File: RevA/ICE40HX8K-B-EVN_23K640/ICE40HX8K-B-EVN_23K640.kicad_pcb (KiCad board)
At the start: 2 copper layers, 50.8 x 17.4 mm, 19 parts, among them J1 2x20_Socket, U0 23K640, U1 23K640, U2 23K640, U3 23K640, U4 23K640, U5 23K640, U6 23K640, U7 23K640

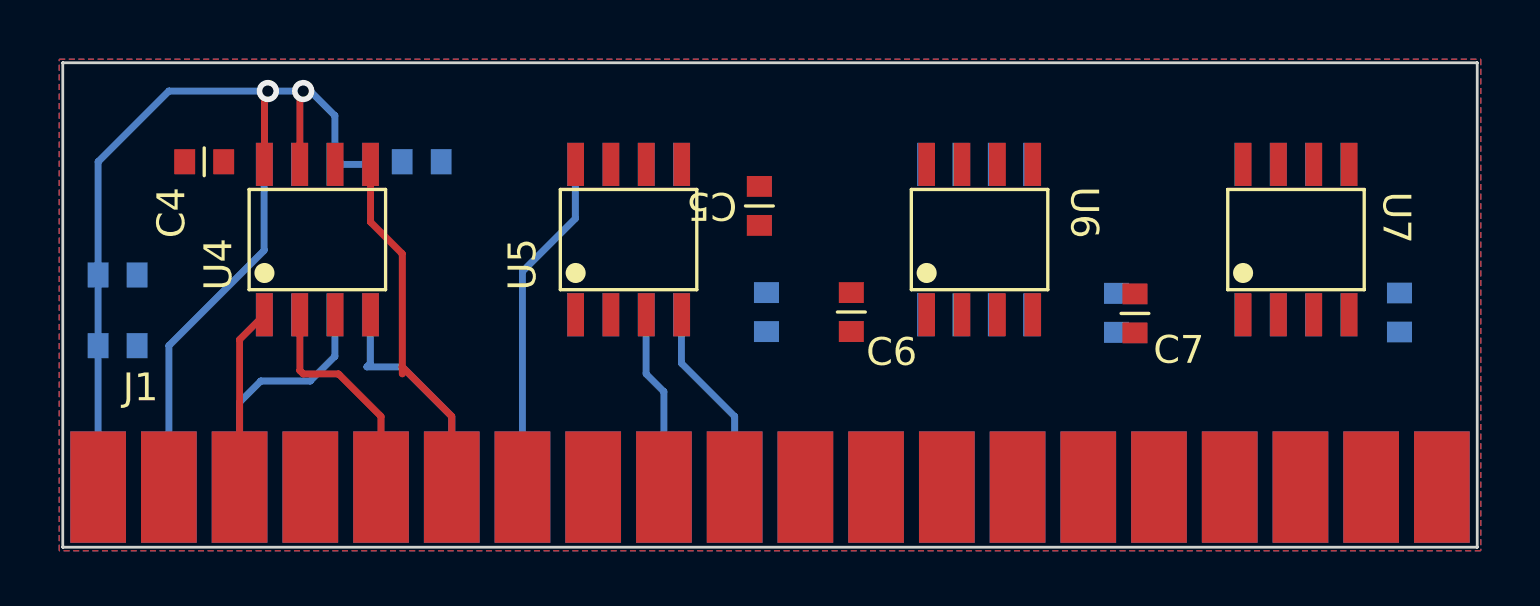
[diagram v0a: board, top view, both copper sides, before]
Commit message: routed
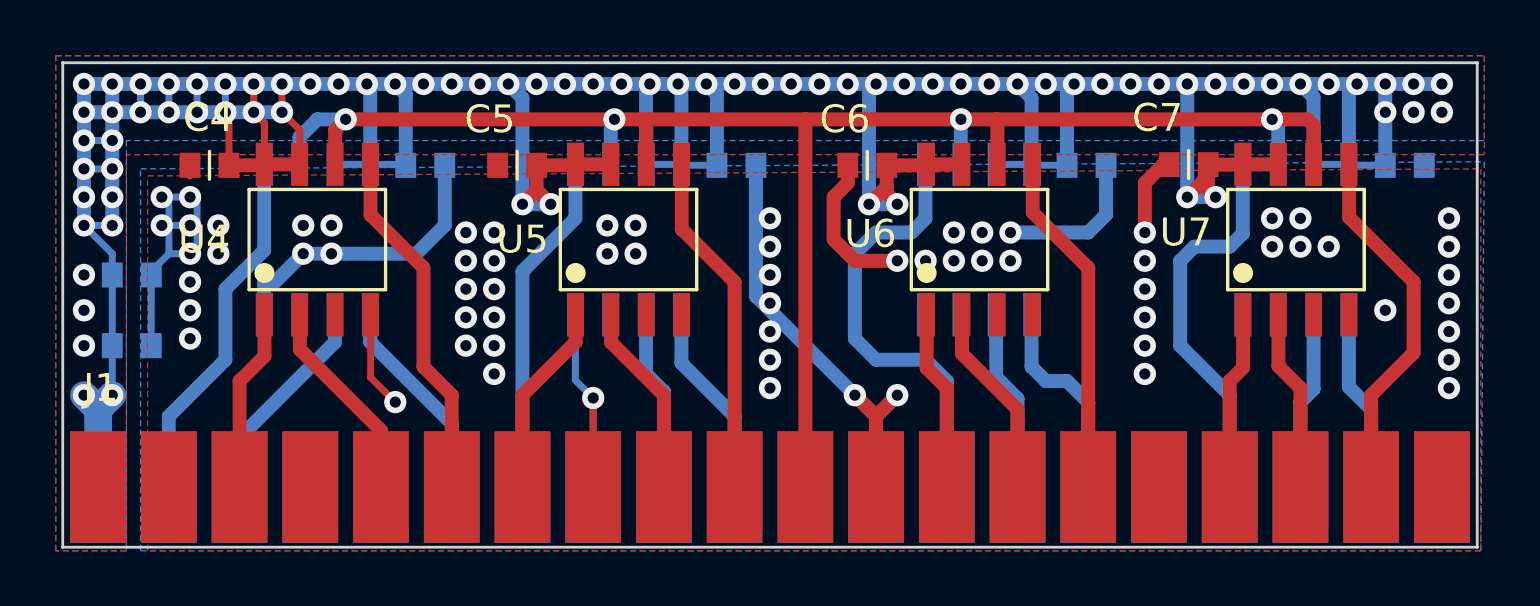
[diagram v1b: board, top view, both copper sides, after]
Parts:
- moved C5 9.65 mm to (80.4, 112.9), turned to 0 degrees
- moved C7 6.17 mm to (104.5, 112.9), turned to 0 degrees
- moved C3 6.05 mm to (113.7, 112.9), turned to 180 degrees
- moved C2 6.01 mm to (102.2, 112.9), turned to 180 degrees
- moved C1 5.98 mm to (89.7, 112.9), turned to 180 degrees
- moved C6 5.97 mm to (93.0, 112.9), turned to 0 degrees
- moved C8 0.51 mm to (67.9, 116.8)
- moved C9 0.51 mm to (67.9, 119.4)
- moved C4 0.23 mm to (69.3, 112.9)
- moved C0 0.18 mm to (78.5, 112.9)
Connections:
- J1 pad 25: /SI_6 -> /nCS_6
- J1 pad 26: /nCS_2 -> /SI_2
- J1 pad 29: /nCS_6 -> /SI_6
- J1 pad 30: /SI_2 -> /nCS_2
- J1 pad 33: /SI_7 -> /nCS_7
- J1 pad 34: /nCS_3 -> /SI_3
- J1 pad 37: /nCS_7 -> /SI_7
- J1 pad 38: /SI_3 -> /nCS_3
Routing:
- net +3V3: track 30.0 -> 190.2 mm, vias 2 -> 79
- net GND: track 0.00 -> 73.5 mm, vias 0 -> 67
- net Net-(J1-Pad21): track 0.00 -> 62.4 mm, vias 0 -> 4
- net /SI_2: track 0.00 -> 15.8 mm
- net /SI_3: track 0.00 -> 14.0 mm
- net /SI_7: track 0.00 -> 13.2 mm
- net /SI_6: track 0.00 -> 12.4 mm
- net /SI_5: track 0.00 -> 12.4 mm
- net /nCS_2: track 0.00 -> 7.48 mm
- net /S0_6: track 0.00 -> 7.02 mm
- net /nCS_5: track 0.00 -> 6.98 mm
- net /S0_5: track 0.00 -> 6.98 mm
- net /nCS_3: track 0.00 -> 6.52 mm
- net /S0_7: track 0.00 -> 6.52 mm
- net /S0_2: track 0.00 -> 6.51 mm
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- added copper zone on B.Cu, net +3V3
- added copper zone on F.Cu, net +3V3
